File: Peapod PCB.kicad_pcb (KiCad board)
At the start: 2 copper layers, 72.5 x 29 mm, 24 parts, among them J1 CONN_01X01, J3 CONN_01X06, J5 CONN_01X01, J6 CONN_01X01, J7 CONN_01X02, U1 ESP8266

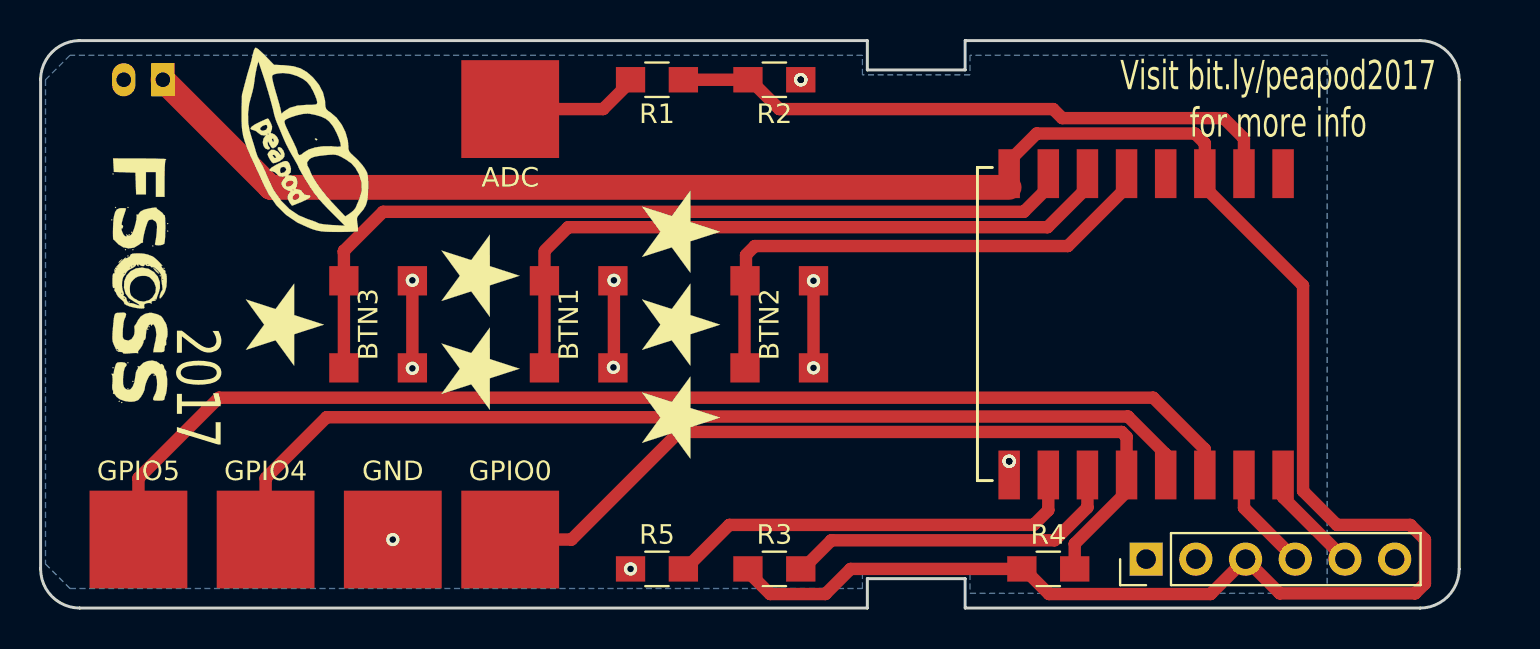
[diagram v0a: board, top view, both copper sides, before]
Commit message: making revisions to design
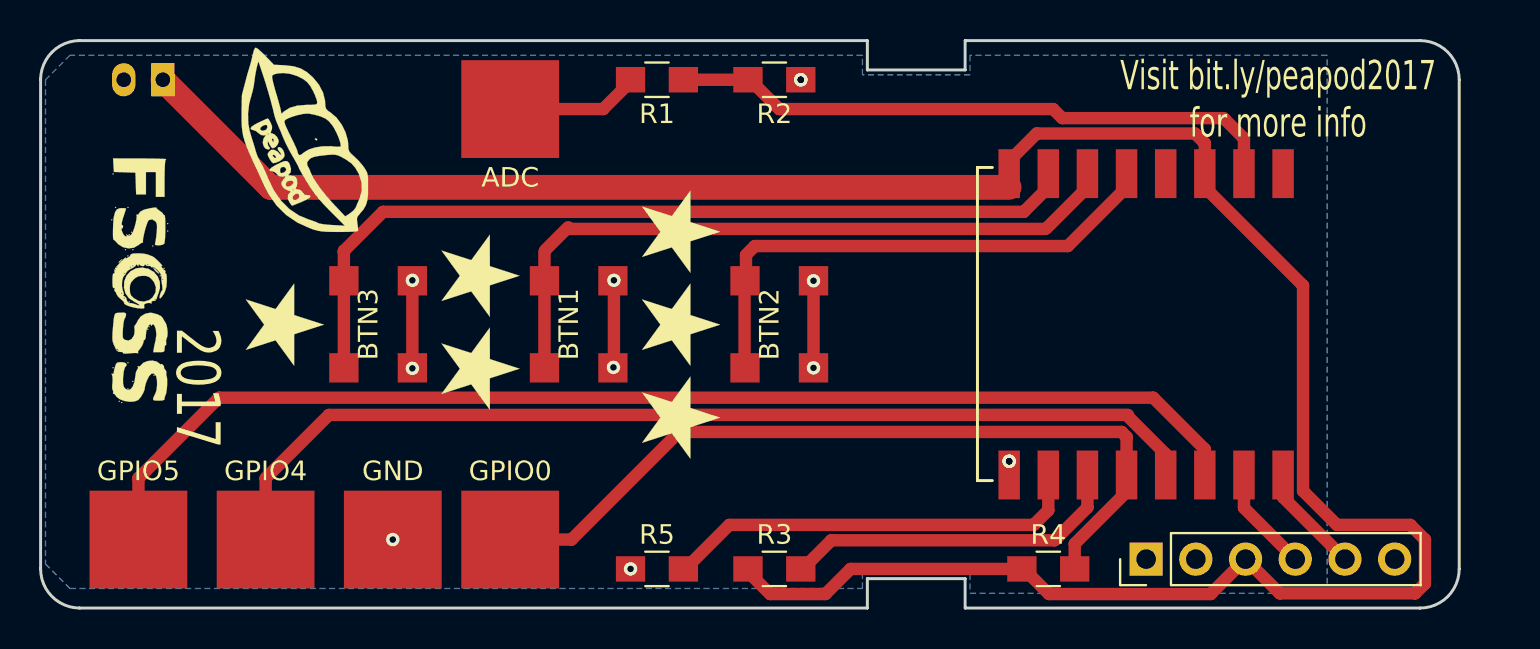
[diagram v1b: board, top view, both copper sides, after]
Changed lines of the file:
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@@
-(kicad_pcb (version 4) (host pcbnew 4.0.4-1.fc24-product)
+(kicad_pcb (version 4) (host pcbnew 4.0.5+dfsg1-4)
   (general
     (links 34)
     (no_connects 1)
-    (area 96.424999 71.924999 169.075001 101.075001)
+    (area 96.424999 30.163 223.01181 103.485733)
     (thickness 1.6002)
     (drawings 32)
-    (tracks 103)
+    (tracks 102)
     (zones 0)
     (modules 24)
@@
   )
   (setup
-    (last_trace_width 0.1524)
+    (last_trace_width 0.381)
     (user_trace_width 0.381)
     (user_trace_width 0.4)
@@
   (via (at 146 93.5) (size 0.6858) (drill 0.3302) (layers F.Cu B.Cu) (net 2))
   (via (at 126.65 99) (size 0.6858) (drill 0.3302) (layers F.Cu B.Cu) (net 2))
-  (segment (start 150 79.5) (end 147.962589 81.537411) (width 0.635) (layer F.Cu) (net 3))
-  (segment (start 147.962589 81.537411) (end 123.462589 81.537411) (width 0.635) (layer F.Cu) (net 3))
+  (segment (start 150 79.5) (end 147.88 81.62) (width 0.635) (layer F.Cu) (net 3))
+  (segment (start 147.8 81.625) (end 123.462589 81.625) (width 0.635) (layer F.Cu) (net 3))
   (segment (start 123.462589 81.537411) (end 122.275 82.725) (width 0.635) (layer F.Cu) (net 3))
   (segment (start 122.25 82.8) (end 122.25 84.185) (width 0.635) (layer F.Cu) (net 3))
@@
   (segment (start 101.5 94.365) (end 105.615 90.25) (width 0.635) (layer F.Cu) (net 10))
   (segment (start 101.5 97.5) (end 101.5 94.365) (width 0.635) (layer F.Cu) (net 10))
+  (segment (start 108 97.5) (end 108 94.365) (width 0.635) (layer F.Cu) (net 11))
+  (segment (start 108 94.365) (end 111.235 91.13) (width 0.635) (layer F.Cu) (net 11))
+  (segment (start 111.235 91.13) (end 128.726255 91.13) (width 0.635) (layer F.Cu) (net 11))
   (segment (start 154 93.136433) (end 154 93.5) (width 0.635) (layer F.Cu) (net 11))
   (segment (start 152.076156 91.212589) (end 154 93.136433) (width 0.635) (layer F.Cu) (net 11))
-  (segment (start 128.808844 91.212589) (end 152.076156 91.212589) (width 0.635) (layer F.Cu) (net 11))
-  (segment (start 128.771433 91.25) (end 128.808844 91.212589) (width 0.635) (layer F.Cu) (net 11))
-  (segment (start 111.115 91.25) (end 128.771433 91.25) (width 0.635) (layer F.Cu) (net 11))
-  (segment (start 108 97.5) (end 108 94.365) (width 0.635) (layer F.Cu) (net 11))
-  (segment (start 108 94.365) (end 111.115 91.25) (width 0.635) (layer F.Cu) (net 11))
+  (segment (start 128.808844 91.125) (end 152.076156 91.125) (width 0.635) (layer F.Cu) (net 11))
+  (segment (start 129.135 92) (end 151.75 92) (width 0.635) (layer F.Cu) (net 12))
   (segment (start 120.5 97.5) (end 123.635 97.5) (width 0.635) (layer F.Cu) (net 12))
   (segment (start 123.635 97.5) (end 129.135 92) (width 0.635) (layer F.Cu) (net 12))
-  (segment (start 129.135 92) (end 151.75 92) (width 0.635) (layer F.Cu) (net 12))
   (segment (start 151.75 92) (end 152 92.25) (width 0.635) (layer F.Cu) (net 12))
   (segment (start 152 92.25) (end 152 93.5) (width 0.635) (layer F.Cu) (net 12))
